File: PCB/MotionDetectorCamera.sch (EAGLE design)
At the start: 186 parts, among them J1 JUMPER-SOLDER, J10 MICROSD-SOCKET, J11 USB-C-JACK, J2 JUMPER-SOLDER, J3 JUMPER-SOLDER, J4 JUMPER-SOLDER, J5 JST-SM02B-SRSS-TB, J6 JUMPER-SOLDER, J7 JUMPER-SOLDER, J8 JUMPER-SOLDER, J9 S-MOUNT-LENS-HOLDERM12LENSES-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, Q1 PMOS-NEXPERIA-SOT1220, Q2 PMOS-NEXPERIA-SOT1220, Q3 PMOS-NEXPERIA-SOT1220, U1 TI-TPS2116, U10 TI-TPS22919DCK, U11 TI-TPS62A01, U13 TI-TPS22919DCK, U14 TI-TPS22919DCK, U15 TI-MSP430FR2422IRHL, U16 NXP-NTB0102, U17 NXP-NTB0102, U18 PANASONIC-EKMB110711X, U19 LATTICE-ICE40HX4K-BG121, U2 DIODESINC-AP7350, U20 WINBOND-W25Q40EW, U21 NEXPERIA-74LVC1G98-OR-INV-INP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, U22 NEXPERIA-74LVC1G98-BUFFER, U23 ON-AR0330CS1C12SPKA0, U24 ALLIANCE-AS4C8M16MSA-6BIN, U25 STM-STM32F730, U26 DIODESINC-DT1446-04V-7, U27 NEXPERIA-74LVC1G98-BUFFER, U3 NEXPERIA-74LVC1G98-NOR, U4 MICROCHIP-MCP7383X, U5 EATON-STN101, U6 TI-TPS62A01, U7 TI-TPS62A01, U9 TI-TPS22919DCK, X1 EPSON-FC-135, X2 SITIME-SIT8021, X3 SITIME-SIT8021

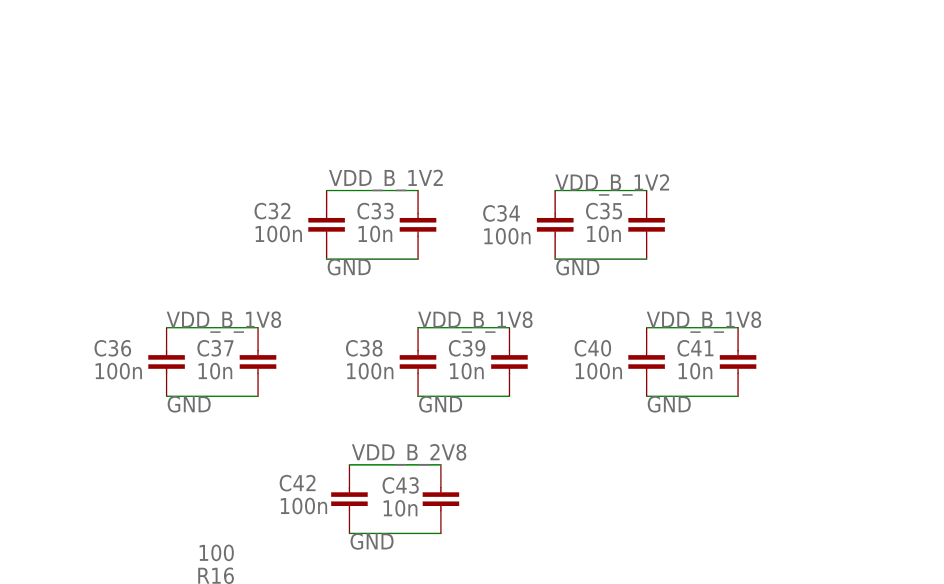
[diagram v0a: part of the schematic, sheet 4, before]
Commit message: Layout progress
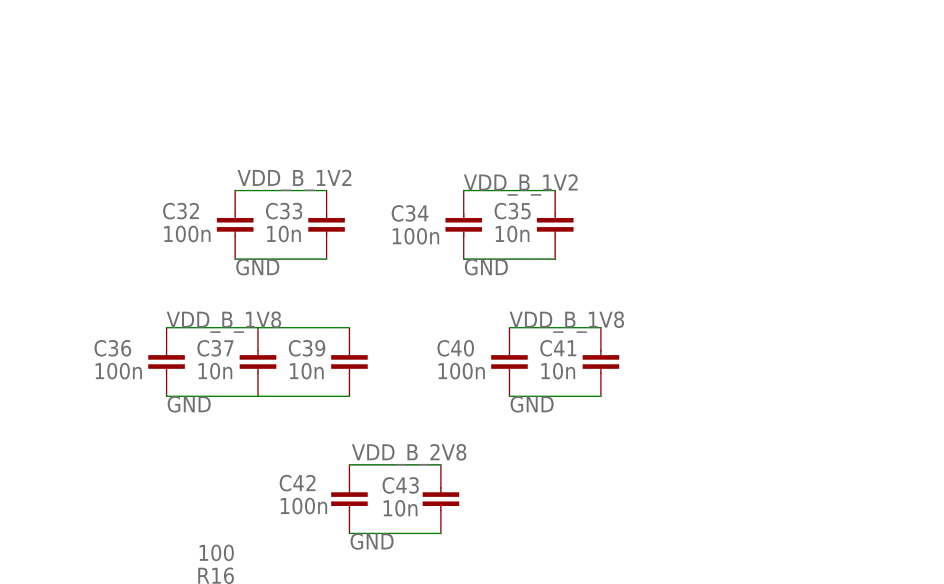
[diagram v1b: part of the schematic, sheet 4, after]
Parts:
- removed C38: 100n, EagleLibrary:CAPACITOR0402
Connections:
- net GND: no longer C38.2
- net VDD_B_1V8: no longer C38.1
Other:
- moved on the sheet: C32, C33, C34, C35, C39, C40, C41
